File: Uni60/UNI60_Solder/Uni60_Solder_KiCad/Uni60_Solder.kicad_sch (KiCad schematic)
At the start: 185 parts, among them J1 Conn_01x04, SW1 SW_Push, SW2 SW_Push, U1 STM32F072CBTx, U2 XC6206PxxxMR, U3 USBLC6-2SC6

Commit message: Update Uni60_Solder.kicad_sch
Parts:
- renumbered KC_RSFT_2.75u to KC_RSFT_2.75u1
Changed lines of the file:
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@@
 		(dnp no)
 		(fields_autoplaced yes)
-		(property "Reference" "KC_RSFT_2.75u"
+		(property "Reference" "KC_RSFT_2.75u1"
 			(at 240.03 90.17 0)
 			(hide yes)
@@
 			(project "Uni60_Solder"
 				(path "/e464f1d1-4c01-4fad-a203-20008a0f30b7"
-					(reference "KC_RSFT_2.75u")
+					(reference "KC_RSFT_2.75u1")
 					(unit 1)
 				)

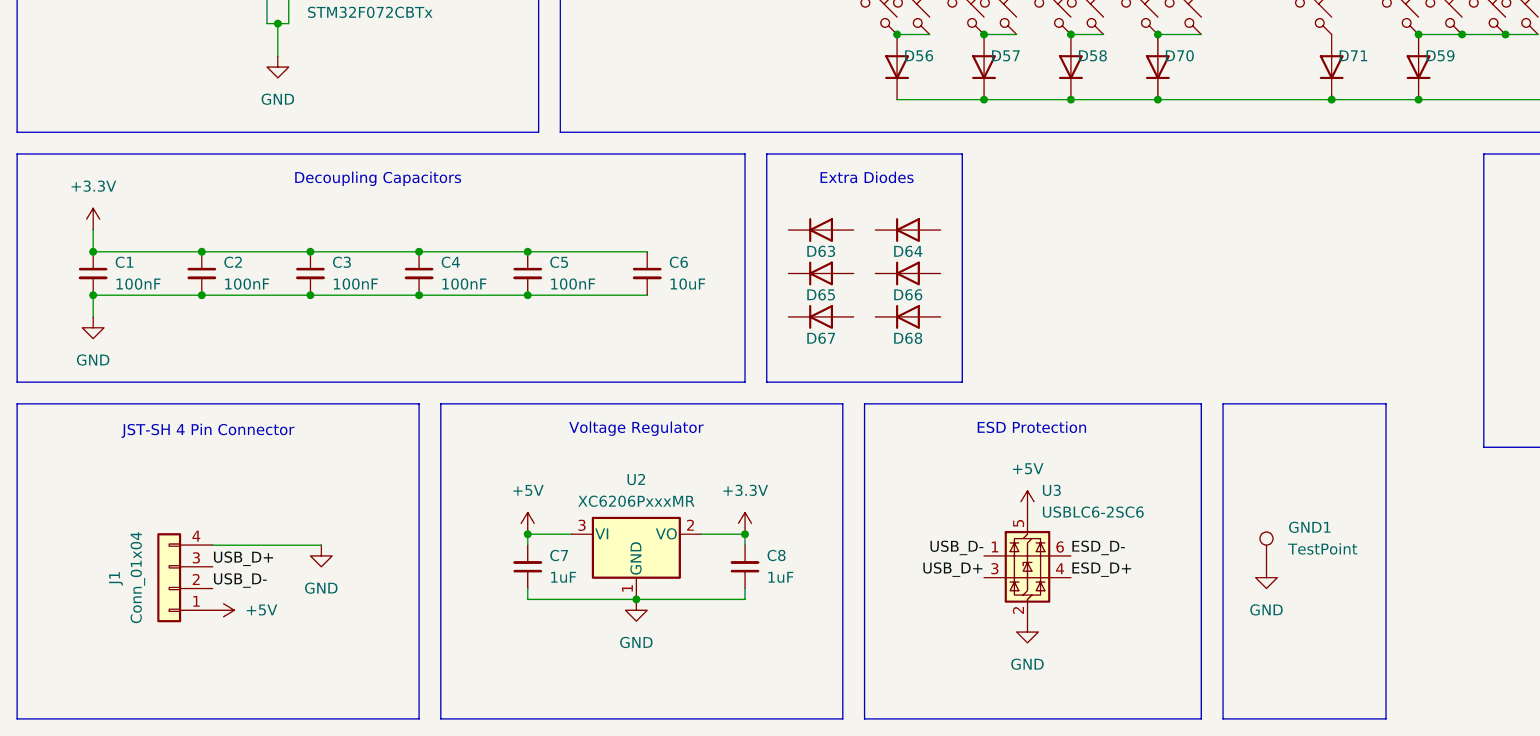
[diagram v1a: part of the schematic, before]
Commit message: Update Uni60_Solder.kicad_sch
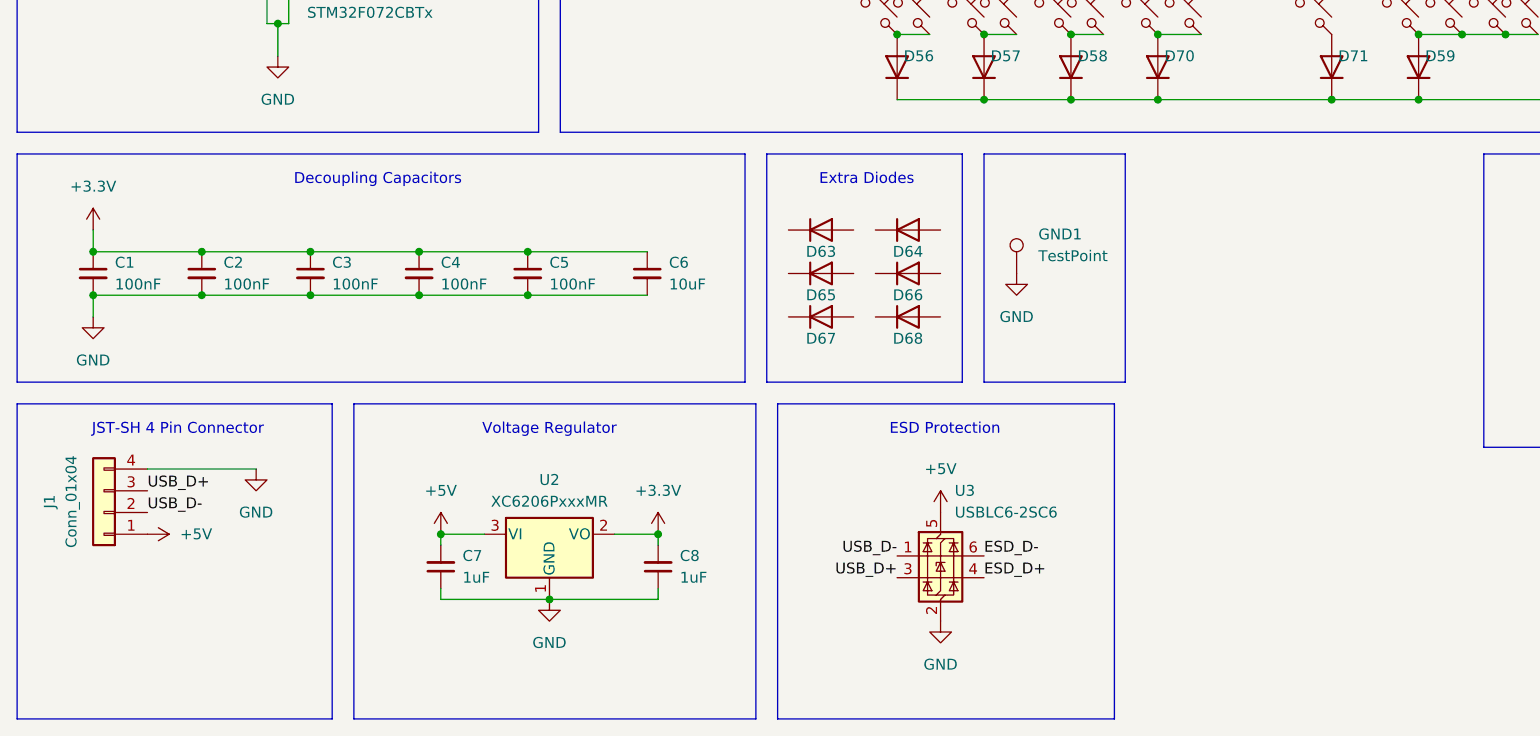
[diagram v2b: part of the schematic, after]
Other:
- title: Velvet Pro Solder PCB v1.0.0 by ShentoBento -> Uni60 PCB v1.0.0 by ShentoBento
- moved on the sheet: C7, C8, GND1, J1, U2, U3

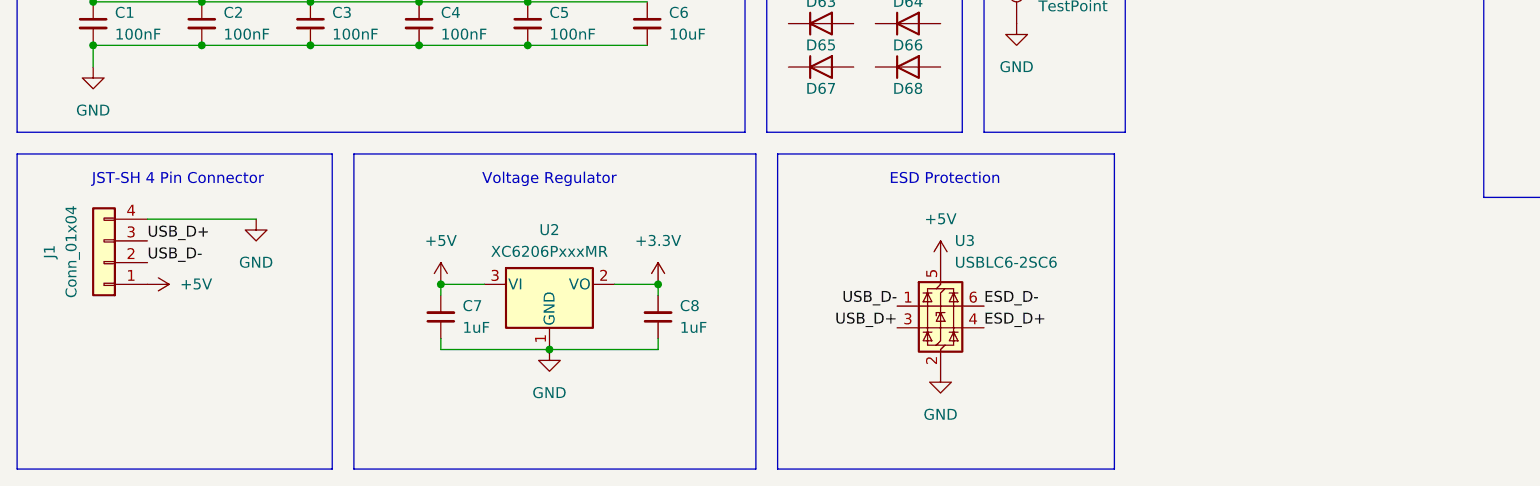
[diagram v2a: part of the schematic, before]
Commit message: idk what changed tbh
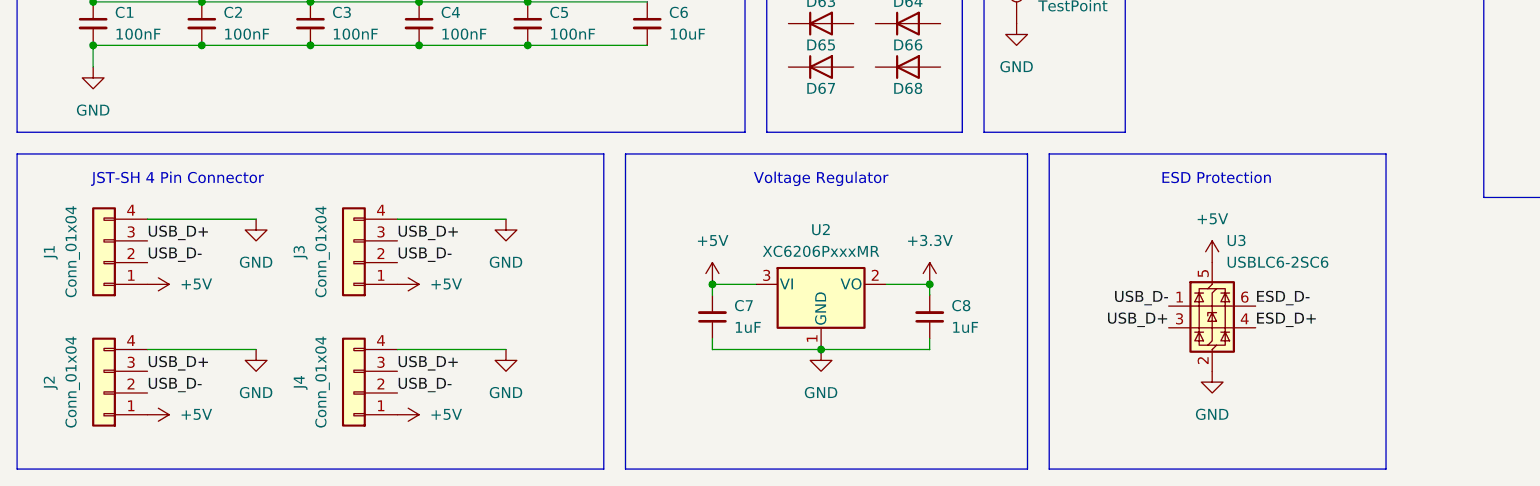
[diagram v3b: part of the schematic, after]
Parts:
- added J2, J3, J4: Conn_01x04, shentobento:JST_SH_1x04, symbol shentobento:Conn_01x04
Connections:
- net +5V: now also J2.1 (Pin_1), J3.1 (Pin_1), J4.1 (Pin_1)
- net GND: now also J2.4 (Pin_4), J3.4 (Pin_4), J4.4 (Pin_4)
- net USB_D+: now also J2.3 (Pin_3), J3.3 (Pin_3), J4.3 (Pin_3)
- net USB_D-: now also J2.2 (Pin_2), J3.2 (Pin_2), J4.2 (Pin_2)
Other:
- moved on the sheet: C7, C8, U2, U3
